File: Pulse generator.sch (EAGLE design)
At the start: 8 parts, among them U1 CD4093BEN14

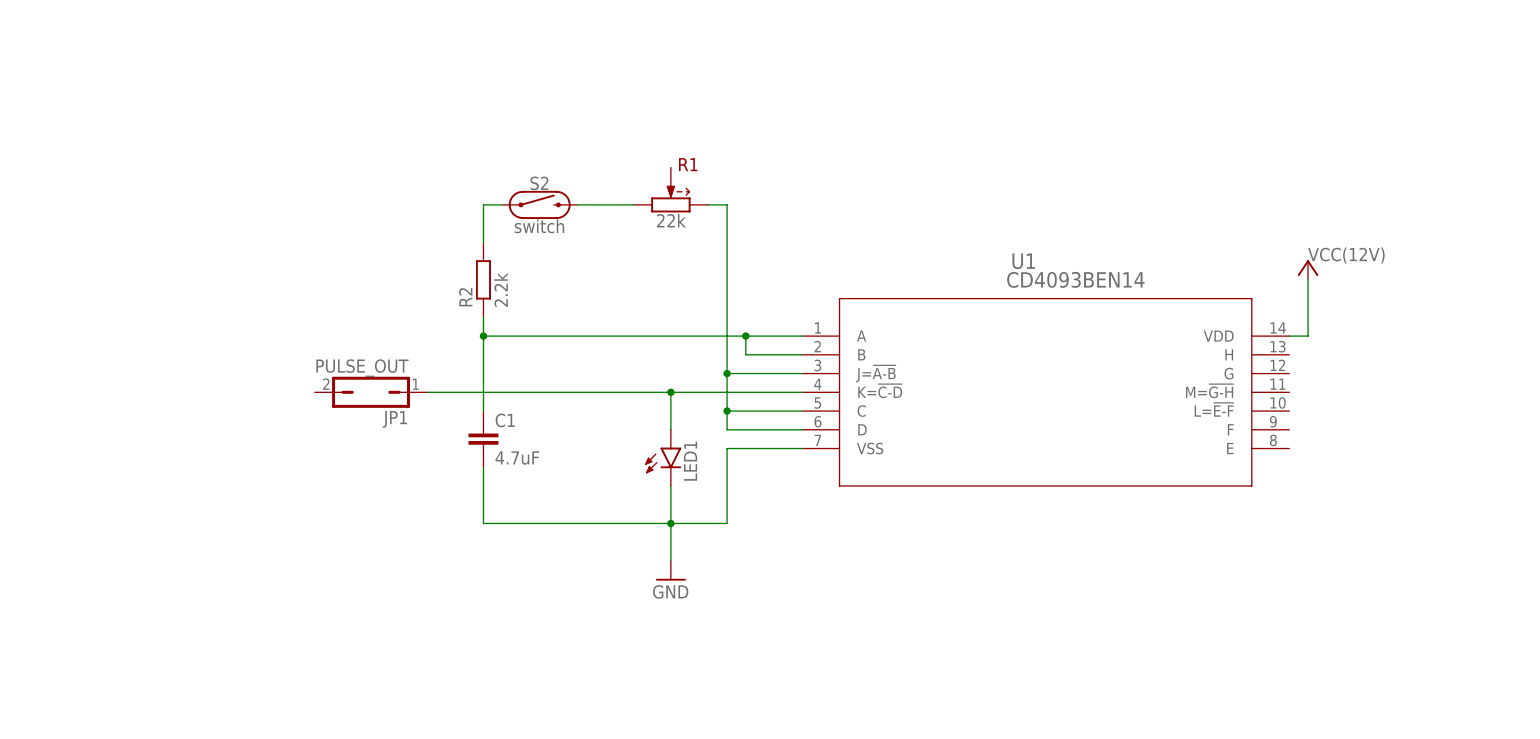
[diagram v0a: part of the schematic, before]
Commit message: Add files via upload
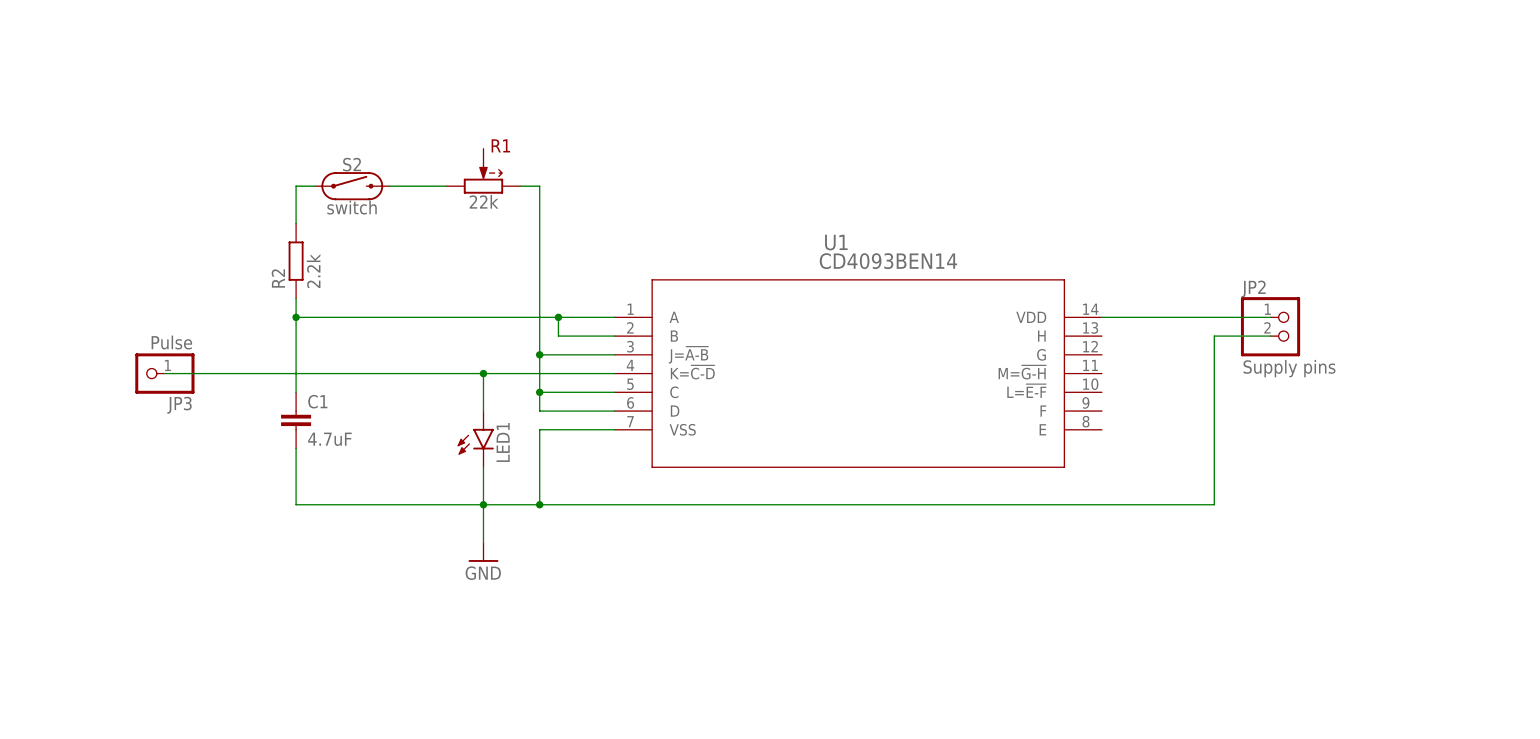
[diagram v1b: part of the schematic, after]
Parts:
- removed JP1: PULSE_OUT, jumper:JP1Q
- added JP2: Supply pins, pinhead:PINHD-1X2
- added JP3: Pulse, pinhead:PINHD-1X1
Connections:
- removed net VCC: U1.VDD
- new net N$1: JP2.1, U1.VDD
- net GND: now also JP2.2
- net N$7: now also JP3.1; no longer JP1.1
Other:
- moved on the sheet: C1, LED1, R1, R2, S2, U1
